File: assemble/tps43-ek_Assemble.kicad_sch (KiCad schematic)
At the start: 14 parts, among them SW1 SW_PUSH, SW2 SW_PUSH, SW3 SW_PUSH, SW4 SW_PUSH, SW5 RotaryEncoder, U1 RP2040-Zero

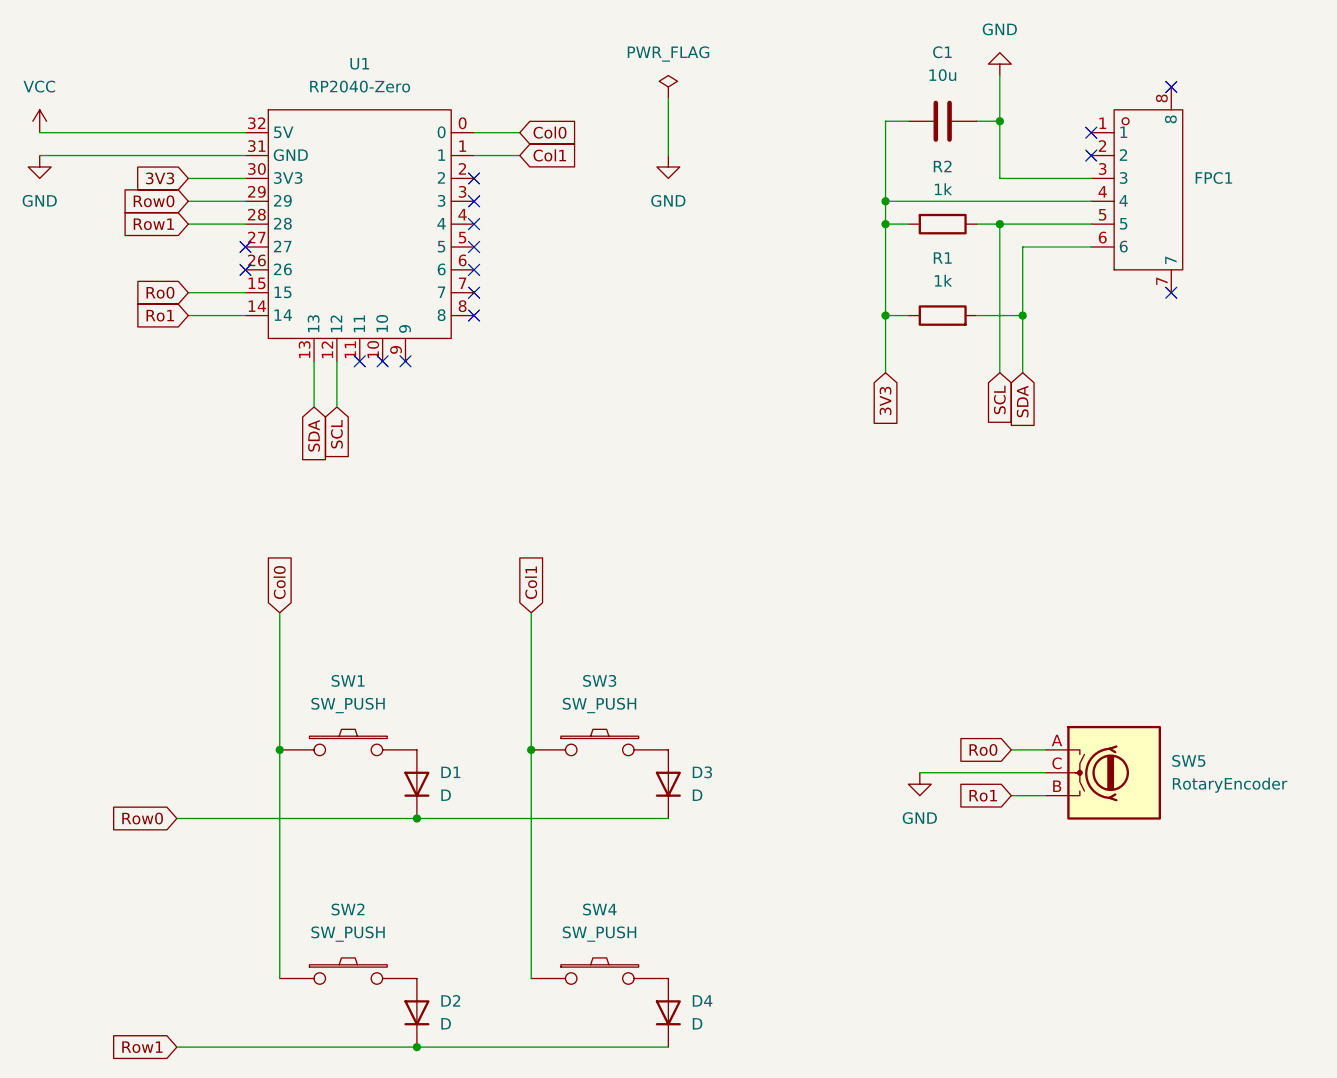
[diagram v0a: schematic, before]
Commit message: 20251130
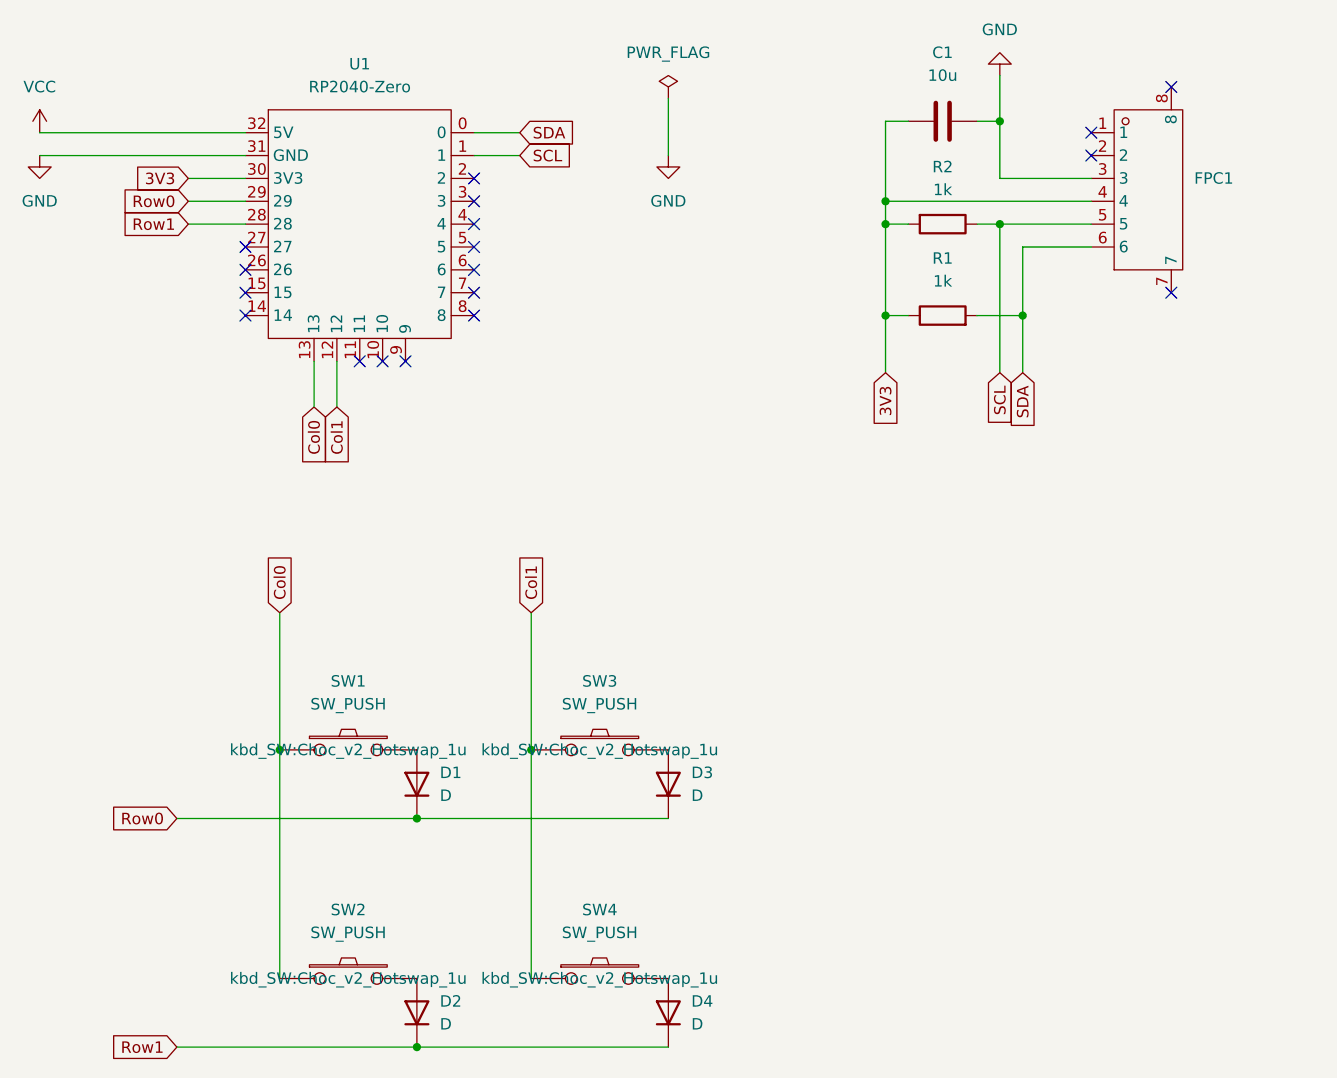
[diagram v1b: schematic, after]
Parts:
- removed SW5: RotaryEncoder, symbol Device:RotaryEncoder
- C1: footprint (none) -> Capacitor_SMD:C_0201_0603Metric
- D1, D2, D3, D4: footprint (none) -> kbd_Parts:Diode_TH_SMD
- FPC1: footprint ProLib_pcs_2025-11-23:FPC-SMD_6P-P0.50_XUNPU_FPC-05F-6PH20 -> Connector_FFC-FPC:FPC-6p-P0.5mm
- R1, R2: footprint (none) -> Resistor_SMD:R_0402_1005Metric
- SW1, SW2, SW3, SW4: footprint (none) -> kbd_SW:Choc_v2_Hotswap_1u
- U1: footprint (none) -> isw-kbd:RP2040-Zero
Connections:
- net Col0: now also U1.13; no longer U1.0
- net Col1: now also U1.12; no longer U1.1
- net SCL: now also U1.1; no longer U1.12
- net SDA: now also U1.0; no longer U1.13
- net Ro0: no longer names the net of U1.15
- net Ro1: no longer names the net of U1.14
- no-connect marks 16 -> 18

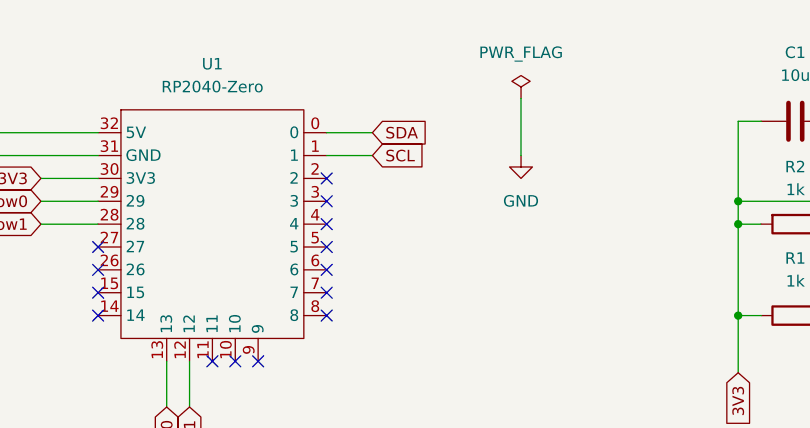
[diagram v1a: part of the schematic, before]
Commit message: 2025-12-02
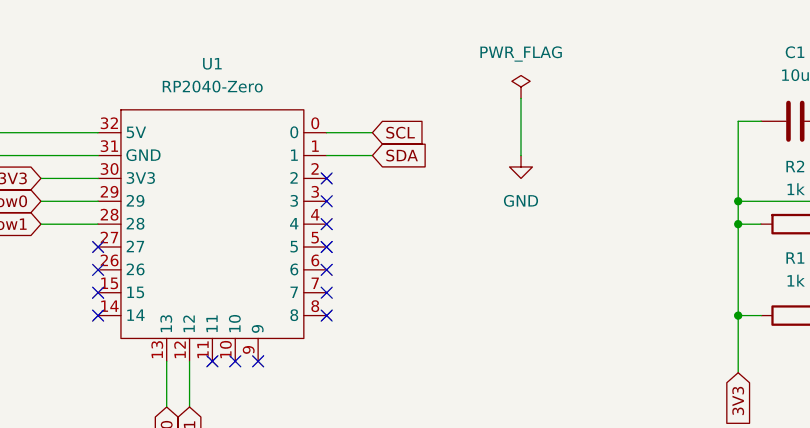
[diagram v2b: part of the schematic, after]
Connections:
- net SCL: now also U1.0; no longer U1.1
- net SDA: now also U1.1; no longer U1.0
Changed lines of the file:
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@@
+		)
+	)
+	(global_label "SDA"
+		(shape input)
+		(at 69.85 29.21 0)
+		(fields_autoplaced yes)
+		(effects
+			(font
+				(size 1.27 1.27)
+			)
+			(justify left)
+		)
+		(property "Intersheetrefs" "${INTERSHEET_REFS}"
+			(at 77.1289 29.21 0)
+			(effects
+				(font
+					(size 1.27 1.27)
+				)
+				(justify left)
+				(hide yes)
+			)
+		)
+	)
+	(global_label "Col1"
+		(shape input)
+		(at 71.12 80.01 90)
+		(fields_autoplaced yes)
+		(effects
+			(font
+				(size 1.27 1.27)
+			)
+			(justify left)
+		)
+		(property "Intersheetrefs" "${INTERSHEET_REFS}"
+			(at 71.12 72.7311 90)
+			(effects
+				(font
+					(size 1.27 1.27)
+				)
+				(justify left)
+				(hide yes)
+			)
 		)
 	)
 	(global_label "SCL"
 		(shape input)
-		(at 69.85 29.21 0)
-		(fields_autoplaced yes)
-		(effects
-			(font
-				(size 1.27 1.27)
-			)
-			(justify left)
-		)
-		(property "Intersheetrefs" "${INTERSHEET_REFS}"
-			(at 77.1289 29.21 0)
-			(effects
-				(font
-					(size 1.27 1.27)
-				)
-				(justify left)
+		(at 123.19 53.34 270)
+		(fields_autoplaced yes)
+		(effects
+			(font
+				(size 1.27 1.27)
+			)
+			(justify right)
+		)
+		(property "Intersheetrefs" "${INTERSHEET_REFS}"
+			(at 123.19 59.8328 90)
+			(effects
+				(font
+					(size 1.27 1.27)
+				)
+				(justify right)
+				(hide yes)
+			)
+		)
+	)
+	(global_label "Col0"
+		(shape input)
+		(at 46.99 57.15 270)
+		(fields_autoplaced yes)
+		(effects
+			(font
+				(size 1.27 1.27)
+			)
+			(justify right)
+		)
+		(property "Intersheetrefs" "${INTERSHEET_REFS}"
+			(at 46.99 63.7033 90)
+			(effects
+				(font
+					(size 1.27 1.27)
+				)
+				(justify right)
+				(hide yes)
+			)
+		)
+	)
+	(global_label "3V3"
+		(shape input)
+		(at 110.49 53.34 270)
+		(fields_autoplaced yes)
+		(effects
+			(font
+				(size 1.27 1.27)
+			)
+			(justify right)
+		)
+		(property "Intersheetrefs" "${INTERSHEET_REFS}"
+			(at 110.49 59.8328 90)
+			(effects
+				(font
+					(size 1.27 1.27)
+				)
+				(justify right)
+				(hide yes)
+			)
+		)
+	)
+	(global_label "SDA"
+		(shape input)
+		(at 125.73 53.34 270)
+		(fields_autoplaced yes)
+		(effects
+			(font
+				(size 1.27 1.27)
+			)
+			(justify right)
+		)
+		(property "Intersheetrefs" "${INTERSHEET_REFS}"
+			(at 125.73 59.8933 90)
+			(effects
+				(font
+					(size 1.27 1.27)
+				)
+				(justify right)
 				(hide yes)
 			)
@@
 	(global_label "Col1"
 		(shape input)
-		(at 71.12 80.01 90)
-		(fields_autoplaced yes)
-		(effects
-			(font
-				(size 1.27 1.27)
-			)
-			(justify left)
-		)
-		(property "Intersheetrefs" "${INTERSHEET_REFS}"
-			(at 71.12 72.7311 90)
-			(effects
-				(font
-					(size 1.27 1.27)
-				)
-				(justify left)
+		(at 49.53 57.15 270)
+		(fields_autoplaced yes)
+		(effects
+			(font
+				(size 1.27 1.27)
+			)
+			(justify right)
+		)
+		(property "Intersheetrefs" "${INTERSHEET_REFS}"
+			(at 49.53 63.6428 90)
+			(effects
+				(font
+					(size 1.27 1.27)
+				)
+				(justify right)
+				(hide yes)
+			)
+		)
+	)
+	(global_label "Row1"
+		(shape input)
+		(at 31.75 128.27 180)
+		(fields_autoplaced yes)
+		(effects
+			(font
+				(size 1.27 1.27)
+			)
+			(justify right)
+		)
+		(property "Intersheetrefs" "${INTERSHEET_REFS}"
+			(at 23.8058 128.27 0)
+			(effects
+				(font
+					(size 1.27 1.27)
+				)
+				(justify right)
+				(hide yes)
+			)
+		)
+	)
+	(global_label "3V3"
+		(shape input)
+		(at 33.02 31.75 180)
+		(fields_autoplaced yes)
+		(effects
+			(font
+				(size 1.27 1.27)
+			)
+			(justify right)
+		)
+		(property "Intersheetrefs" "${INTERSHEET_REFS}"
+			(at 26.6482 31.75 0)
+			(effects
+				(font
+					(size 1.27 1.27)
+				)
+				(justify right)
+				(hide yes)
+			)
+		)
+	)
+	(global_label "Row0"
+		(shape input)
+		(at 31.75 102.87 180)
+		(fields_autoplaced yes)
+		(effects
+			(font
+				(size 1.27 1.27)
+			)
+			(justify right)
+		)
+		(property "Intersheetrefs" "${INTERSHEET_REFS}"
+			(at 23.8058 102.87 0)
+			(effects
+				(font
+					(size 1.27 1.27)
+				)
+				(justify right)
 				(hide yes)
 			)
@@
 	(global_label "SCL"
 		(shape input)
-		(at 123.19 53.34 270)
-		(fields_autoplaced yes)
-		(effects
-			(font
-				(size 1.27 1.27)
-			)
-			(justify right)
-		)
-		(property "Intersheetrefs" "${INTERSHEET_REFS}"
-			(at 123.19 59.8328 90)
-			(effects
-				(font
-					(size 1.27 1.27)
-				)
-				(justify right)
-				(hide yes)
-			)
-		)
-	)
-	(global_label "Col0"
-		(shape input)
-		(at 46.99 57.15 270)
-		(fields_autoplaced yes)
-		(effects
-			(font
-				(size 1.27 1.27)
-			)
-			(justify right)
-		)
-		(property "Intersheetrefs" "${INTERSHEET_REFS}"
-			(at 46.99 63.7033 90)
-			(effects
-				(font
-					(size 1.27 1.27)
-				)
-				(justify right)
-				(hide yes)
-			)
-		)
-	)
-	(global_label "3V3"
-		(shape input)
-		(at 110.49 53.34 270)
-		(fields_autoplaced yes)
-		(effects
-			(font
-				(size 1.27 1.27)
-			)
-			(justify right)
-		)
-		(property "Intersheetrefs" "${INTERSHEET_REFS}"
-			(at 110.49 59.8328 90)
-			(effects
-				(font
-					(size 1.27 1.27)
-				)
-				(justify right)
-				(hide yes)
-			)
-		)
-	)
-	(global_label "SDA"
-		(shape input)
-		(at 125.73 53.34 270)
-		(fields_autoplaced yes)
-		(effects
-			(font
-				(size 1.27 1.27)
-			)
-			(justify right)
-		)
-		(property "Intersheetrefs" "${INTERSHEET_REFS}"
-			(at 125.73 59.8933 90)
-			(effects
-				(font
-					(size 1.27 1.27)
-				)
-				(justify right)
-				(hide yes)
-			)
-		)
-	)
-	(global_label "Col1"
-		(shape input)
-		(at 49.53 57.15 270)
-		(fields_autoplaced yes)
-		(effects
-			(font
-				(size 1.27 1.27)
-			)
-			(justify right)
-		)
-		(property "Intersheetrefs" "${INTERSHEET_REFS}"
-			(at 49.53 63.6428 90)
-			(effects
-				(font
-					(size 1.27 1.27)
-				)
-				(justify right)
-				(hide yes)
-			)
-		)
-	)
-	(global_label "Row1"
-		(shape input)
-		(at 31.75 128.27 180)
-		(fields_autoplaced yes)
-		(effects
-			(font
-				(size 1.27 1.27)
-			)
-			(justify right)
-		)
-		(property "Intersheetrefs" "${INTERSHEET_REFS}"
-			(at 23.8058 128.27 0)
-			(effects
-				(font
-					(size 1.27 1.27)
-				)
-				(justify right)
-				(hide yes)
-			)
-		)
-	)
-	(global_label "3V3"
-		(shape input)
-		(at 33.02 31.75 180)
-		(fields_autoplaced yes)
-		(effects
-			(font
-				(size 1.27 1.27)
-			)
-			(justify right)
-		)
-		(property "Intersheetrefs" "${INTERSHEET_REFS}"
-			(at 26.6482 31.75 0)
-			(effects
-				(font
-					(size 1.27 1.27)
-				)
-				(justify right)
-				(hide yes)
-			)
-		)
-	)
-	(global_label "Row0"
-		(shape input)
-		(at 31.75 102.87 180)
-		(fields_autoplaced yes)
-		(effects
-			(font
-				(size 1.27 1.27)
-			)
-			(justify right)
-		)
-		(property "Intersheetrefs" "${INTERSHEET_REFS}"
-			(at 23.8058 102.87 0)
-			(effects
-				(font
-					(size 1.27 1.27)
-				)
-				(justify right)
-				(hide yes)
-			)
-		)
-	)
-	(global_label "SDA"
-		(shape input)
 		(at 69.85 26.67 0)

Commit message: progress 2025-12-04
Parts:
- C1: footprint Capacitor_SMD:C_0201_0603Metric -> Capacitor_SMD:C_0603_1608Metric_Pad1.08x0.95mm_HandSolder
- R1, R2: footprint Resistor_SMD:R_0402_1005Metric -> Resistor_SMD:R_0603_1608Metric_Pad0.98x0.95mm_HandSolder
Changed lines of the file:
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@@
 			)
 		)
-		(property "Footprint" "Resistor_SMD:R_0402_1005Metric"
+		(property "Footprint" "Resistor_SMD:R_0603_1608Metric_Pad0.98x0.95mm_HandSolder"
 			(at 116.84 48.768 90)
 			(effects
@@
 			)
 		)
-		(property "Footprint" "Resistor_SMD:R_0402_1005Metric"
+		(property "Footprint" "Resistor_SMD:R_0603_1608Metric_Pad0.98x0.95mm_HandSolder"
 			(at 116.84 35.052 90)
 			(effects
@@
 			)
 		)
-		(property "Footprint" "Capacitor_SMD:C_0201_0603Metric"
+		(property "Footprint" "Capacitor_SMD:C_0603_1608Metric_Pad1.08x0.95mm_HandSolder"
 			(at 120.65 24.4348 0)
 			(effects
